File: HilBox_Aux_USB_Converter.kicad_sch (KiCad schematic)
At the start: 27 parts, among them J7 USB_C_Plug_USB2.0, J8 Conn_01x04_Pin, U11 USB6B1RL, U12 FT232RL

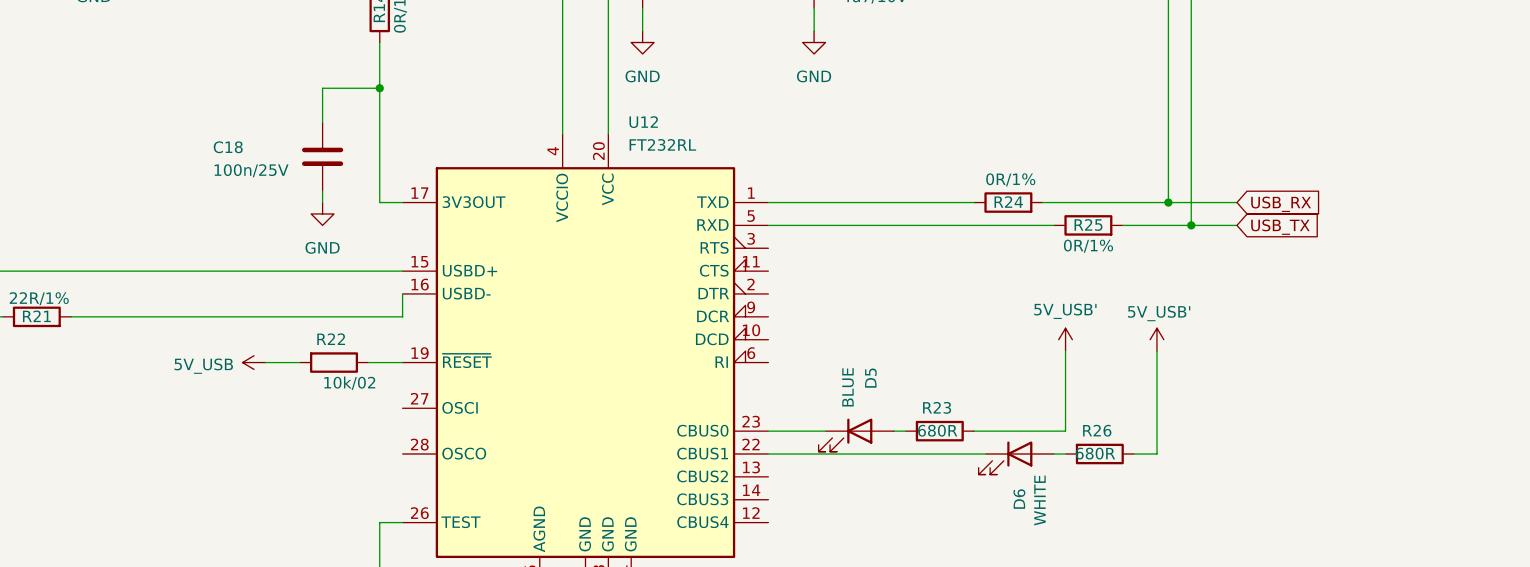
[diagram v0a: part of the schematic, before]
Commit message: Gate finalized! PCB ordered
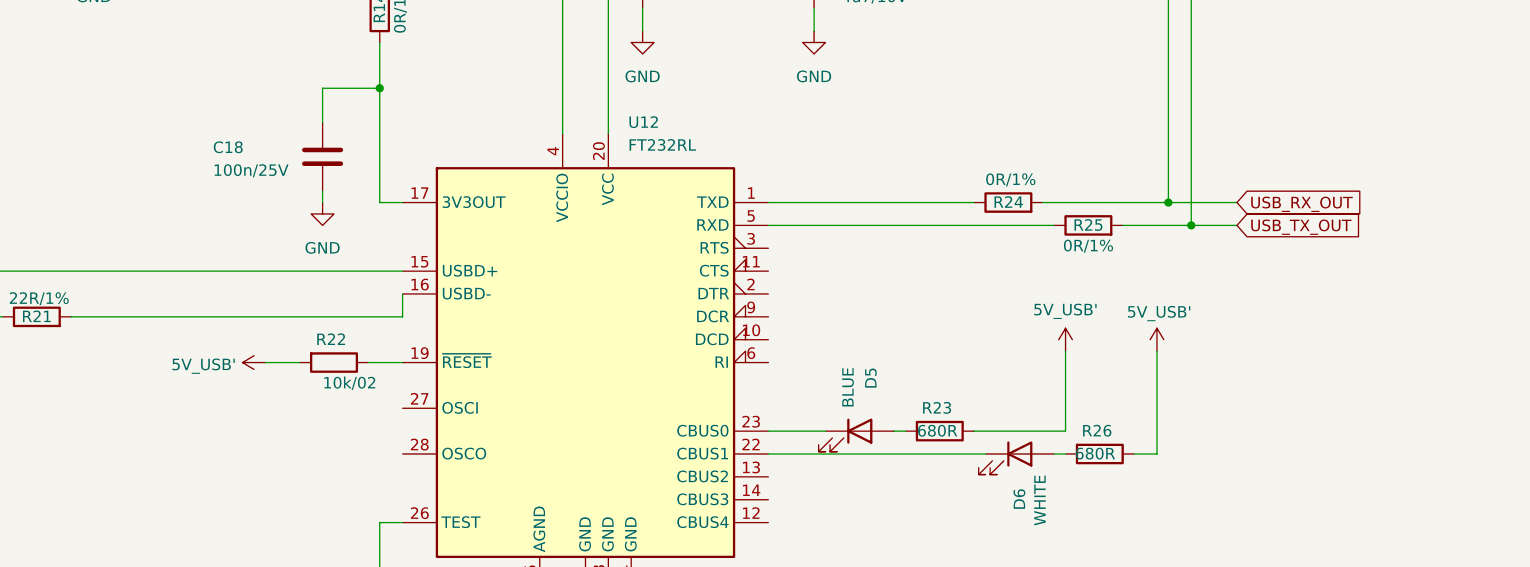
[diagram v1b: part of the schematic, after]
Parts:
- J8: JLC_PN (none) -> C7430360
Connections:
- net 5V_USB is gone; now on net 5V_USB': R22.2
- net USB_RX renamed USB_RX_OUT
- net USB_TX renamed USB_TX_OUT
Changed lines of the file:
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@@
 		)
 	)
-	(global_label "USB_RX"
+	(global_label "USB_RX_OUT"
 		(shape input)
 		(at 252.73 90.17 0)
@@
 		)
 		(property "Intersheetrefs" "${INTERSHEET_REFS}"
-			(at 262.9723 90.17 0)
+			(at 267.5685 90.17 0)
 			(effects
 				(font
@@
 		)
 	)
-	(global_label "USB_TX"
+	(global_label "USB_TX_OUT"
 		(shape input)
 		(at 252.73 92.71 0)
@@
 		)
 		(property "Intersheetrefs" "${INTERSHEET_REFS}"
-			(at 262.6699 92.71 0)
+			(at 267.2661 92.71 0)
 			(effects
 				(font
@@
 			)
 		)
+		(property "JLC_PN" "C7430360"
+			(at 264.16 46.99 0)
+			(effects
+				(font
+					(size 1.27 1.27)
+				)
+				(hide yes)
+			)
+		)
 		(pin "3"
 		)
@@
 			)
 		)
-		(property "Value" "5V_USB"
+		(property "Value" "5V_USB'"
 			(at 137.922 108.204 90)
 			(effects
